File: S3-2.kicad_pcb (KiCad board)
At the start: 2 copper layers, 20.1 x 35.5 mm, 50 parts, among them J1 JST SH1.0, J2 USB_C_Receptacle_USB2.0_16P, J3 JST PH2.0, Q1 AO3401A, Q2 AO3400A, SW1 SW_Push, SW2 SW_Push, SW3 SW_Push_SPDT, U2 ESP32-S3-WROOM-1, U3 ME6211C33M5, U4 TP4057, U5 XC6206P182MR, U6 MPU-9250

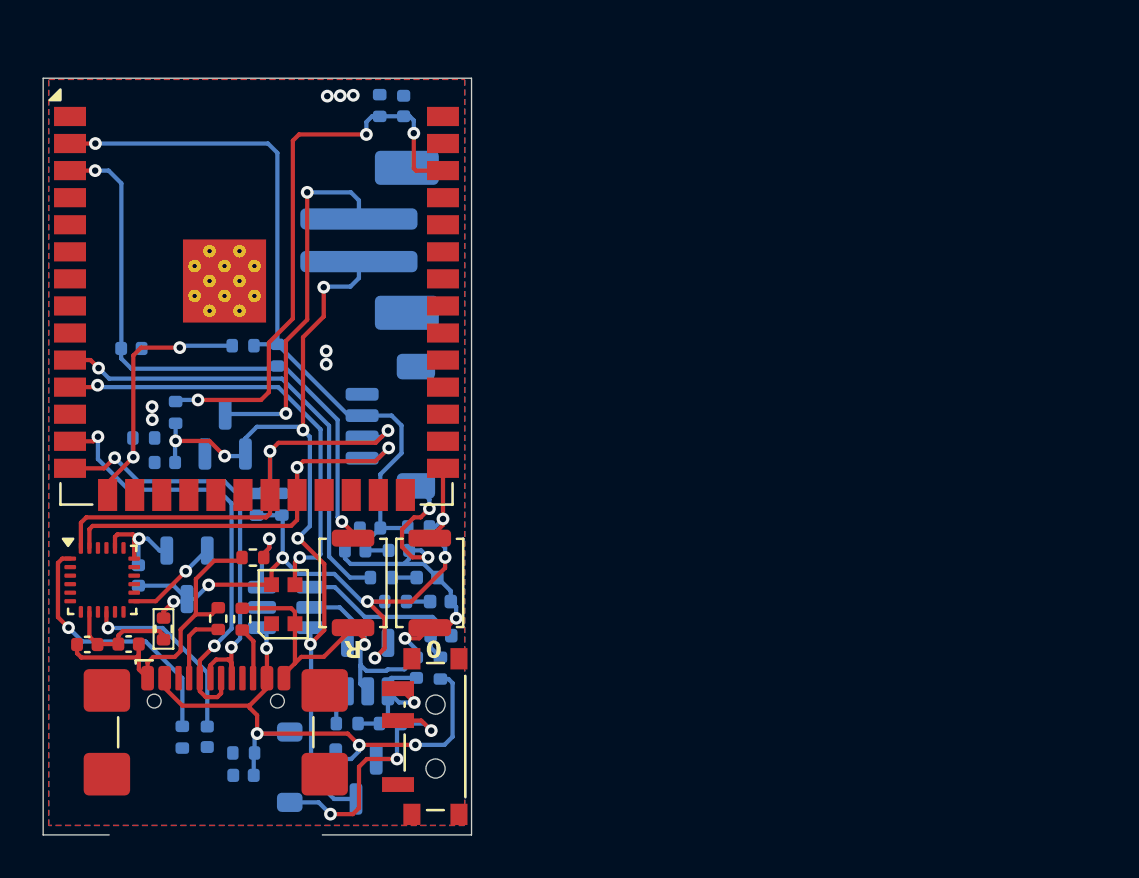
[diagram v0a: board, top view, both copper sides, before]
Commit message: Update Board
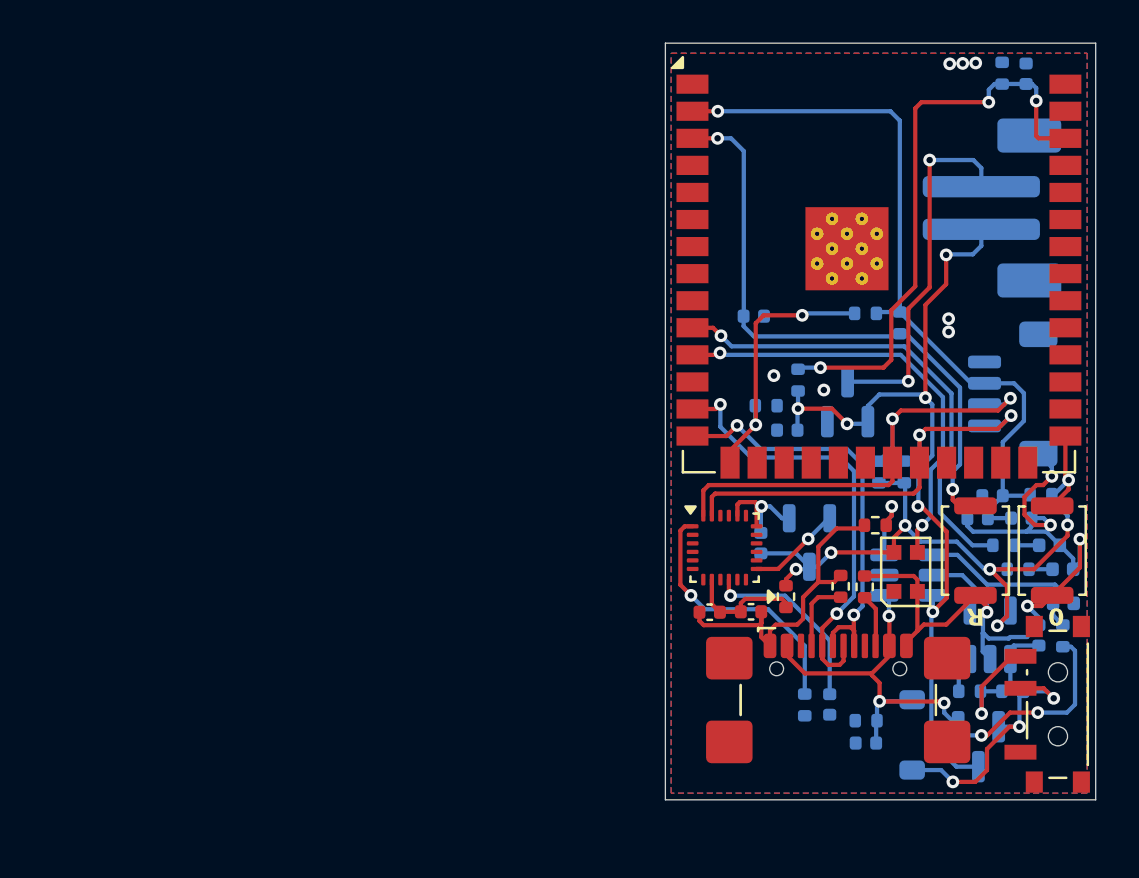
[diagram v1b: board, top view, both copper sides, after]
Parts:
- moved C1 29.2 mm to (62.0, 69.1)
- moved C10 29.2 mm to (63.6, 74.4)
- moved C6 29.2 mm to (74.6, 78.6)
- moved D1 29.2 mm to (69.4, 88.7)
- moved J2 29.2 mm to (66.0, 88.2)
- moved J3 29.2 mm to (73.2, 64.0)
- moved Q1 29.2 mm to (72.5, 89.3)
- moved R1 29.2 mm to (67.3, 88.1)
- moved R10 29.2 mm to (73.7, 79.8)
- moved R2 29.2 mm to (68.9, 69.4)
- moved R3 29.2 mm to (75.5, 77.5)
- moved R4 29.2 mm to (67.2, 69.0)
- moved C13 29.2 mm to (59.9, 83.0)
- moved C11 29.2 mm to (62.3, 79.7)
- moved C12 29.2 mm to (61.9, 83.0)
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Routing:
- net GND: track 60.1 -> 62.6 mm
- net 5V: track 7.04 -> 9.31 mm
- net EN: track 28.2 -> 28.9 mm
- net +5V: track 13.5 -> 12.9 mm
- net VBUS: track 28.2 -> 27.8 mm, vias 4 -> 5
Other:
- board size 20.1 x 35.5 mm -> 20.2 x 35.5 mm
- board text added: "S3-2"
